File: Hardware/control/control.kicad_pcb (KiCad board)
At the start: 2 copper layers, 100 x 100 mm, 65 parts, among them J1 Conn_02x12_Odd_Even

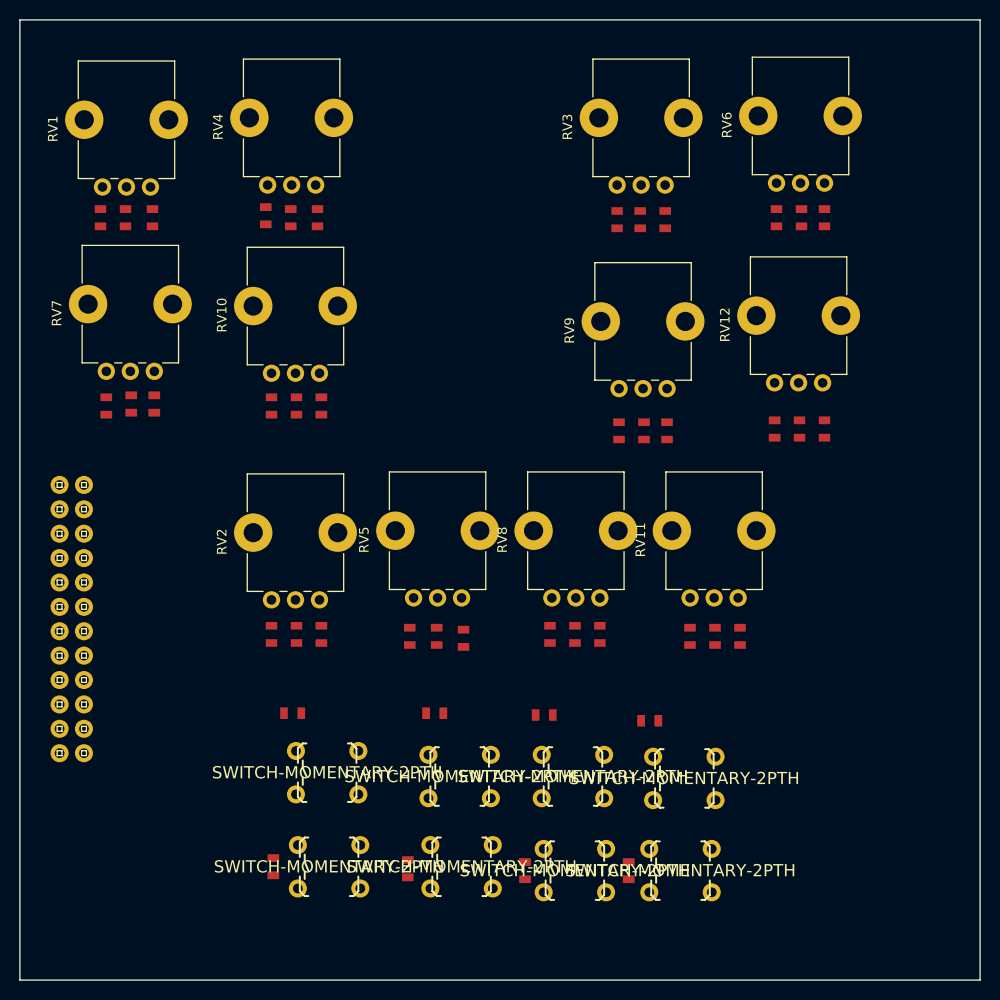
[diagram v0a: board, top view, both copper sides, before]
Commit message: route control board
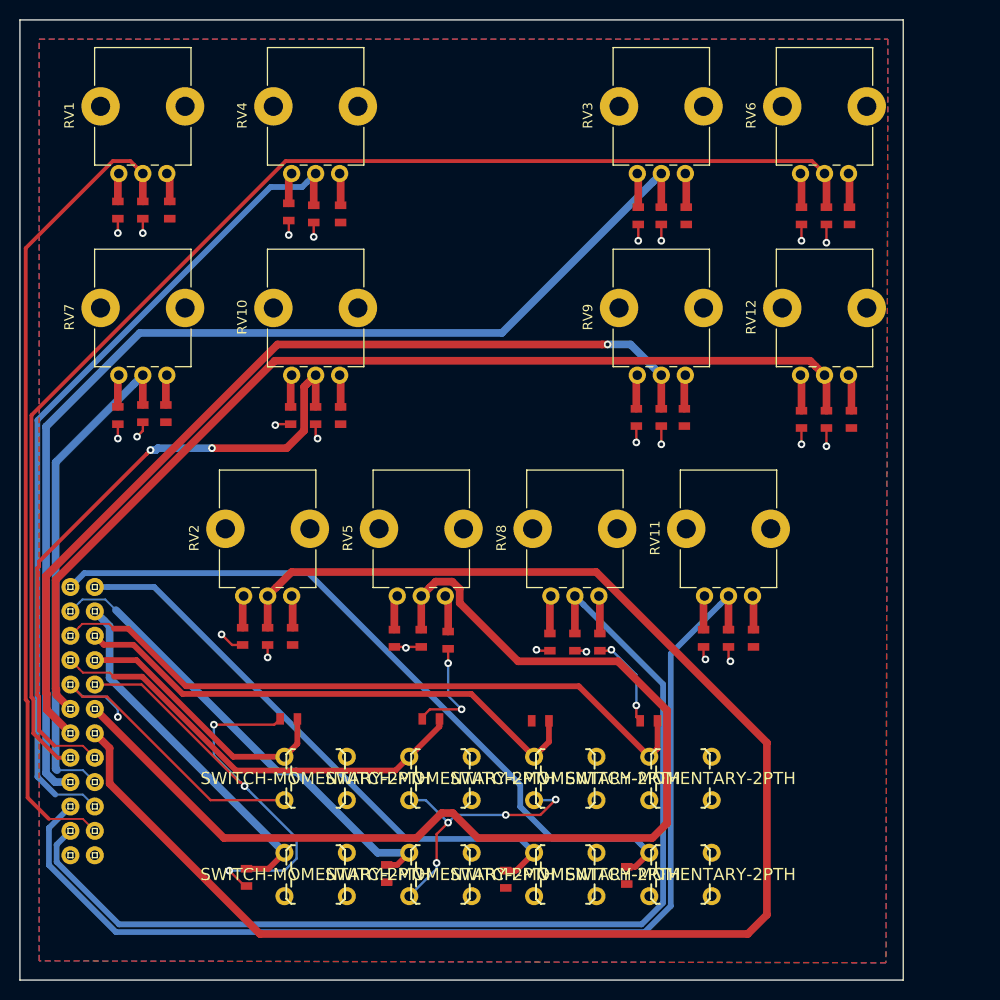
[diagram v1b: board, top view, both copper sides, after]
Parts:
- moved J1 10.7 mm to (6.53, 73.0), turned to 90 degrees
- moved R2 3.01 mm to (23.6, 89.3)
- moved C2 3.01 mm to (25.8, 64.2)
- moved R11 3.01 mm to (28.4, 64.2)
- moved R12 3.01 mm to (23.2, 64.2)
- moved R32 2.97 mm to (81.4, 41.6)
- moved C12 2.97 mm to (84.0, 41.6)
- moved R31 2.97 mm to (86.6, 41.6)
- moved RV2 2.93 mm to (28.3, 60.0)
- moved RV12 2.82 mm to (86.3, 37.0)
- moved RV4 2.77 mm to (33.3, 16.0)
- moved RV6 2.69 mm to (86.3, 16.0)
- moved R19 2.61 mm to (86.4, 20.4)
- moved R20 2.61 mm to (81.4, 20.4)
- moved C6 2.61 mm to (84.0, 20.4)
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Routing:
- net /attack: track 0.00 -> 163.3 mm
- net /lfo_depth: track 0.00 -> 135.8 mm
- net /lfo_rate: track 0.00 -> 117.5 mm
- net /decay: track 0.00 -> 115.8 mm
- net /release: track 0.00 -> 114.1 mm
- net /sustain: track 0.00 -> 110.3 mm
- net /global_lfo_depth: track 0.00 -> 108.0 mm
- net GND: track 0.00 -> 102.1 mm, vias 0 -> 28
- net /global_lfo_rate: track 0.00 -> 96.3 mm, vias 0 -> 1
- net /osc1_waveshape: track 0.00 -> 87.4 mm
- net /osc1_tune: track 0.00 -> 85.1 mm
- net /mod8: track 0.00 -> 77.2 mm
- net 3.3V: track 0.00 -> 76.0 mm, vias 0 -> 7
- net /mod4: track 0.00 -> 70.6 mm
- net /osc2_waveshape: track 0.00 -> 67.6 mm, vias 0 -> 2
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- added copper zone on F.Cu, net 3.3V
- added copper zone on B.Cu, net GND
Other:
- board size 100 x 100 mm -> 92 x 100 mm
